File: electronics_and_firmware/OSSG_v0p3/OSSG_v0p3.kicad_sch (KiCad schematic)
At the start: 71 parts, among them IC1 DW01A, J1 USB_B_Micro, J2 External PDM Mic Input, Q1 FS8205A, Q2 Q_NPN_BEC, Q3 Q_NPN_BEC, SW1 SW_SPST, U1 ESP32-PICO-D4, U2 TP4056, U3 XC6222B331MRG, U4 FT232RQ, U5 APX803L-29SA-7, U6 MP23DB01HPTR

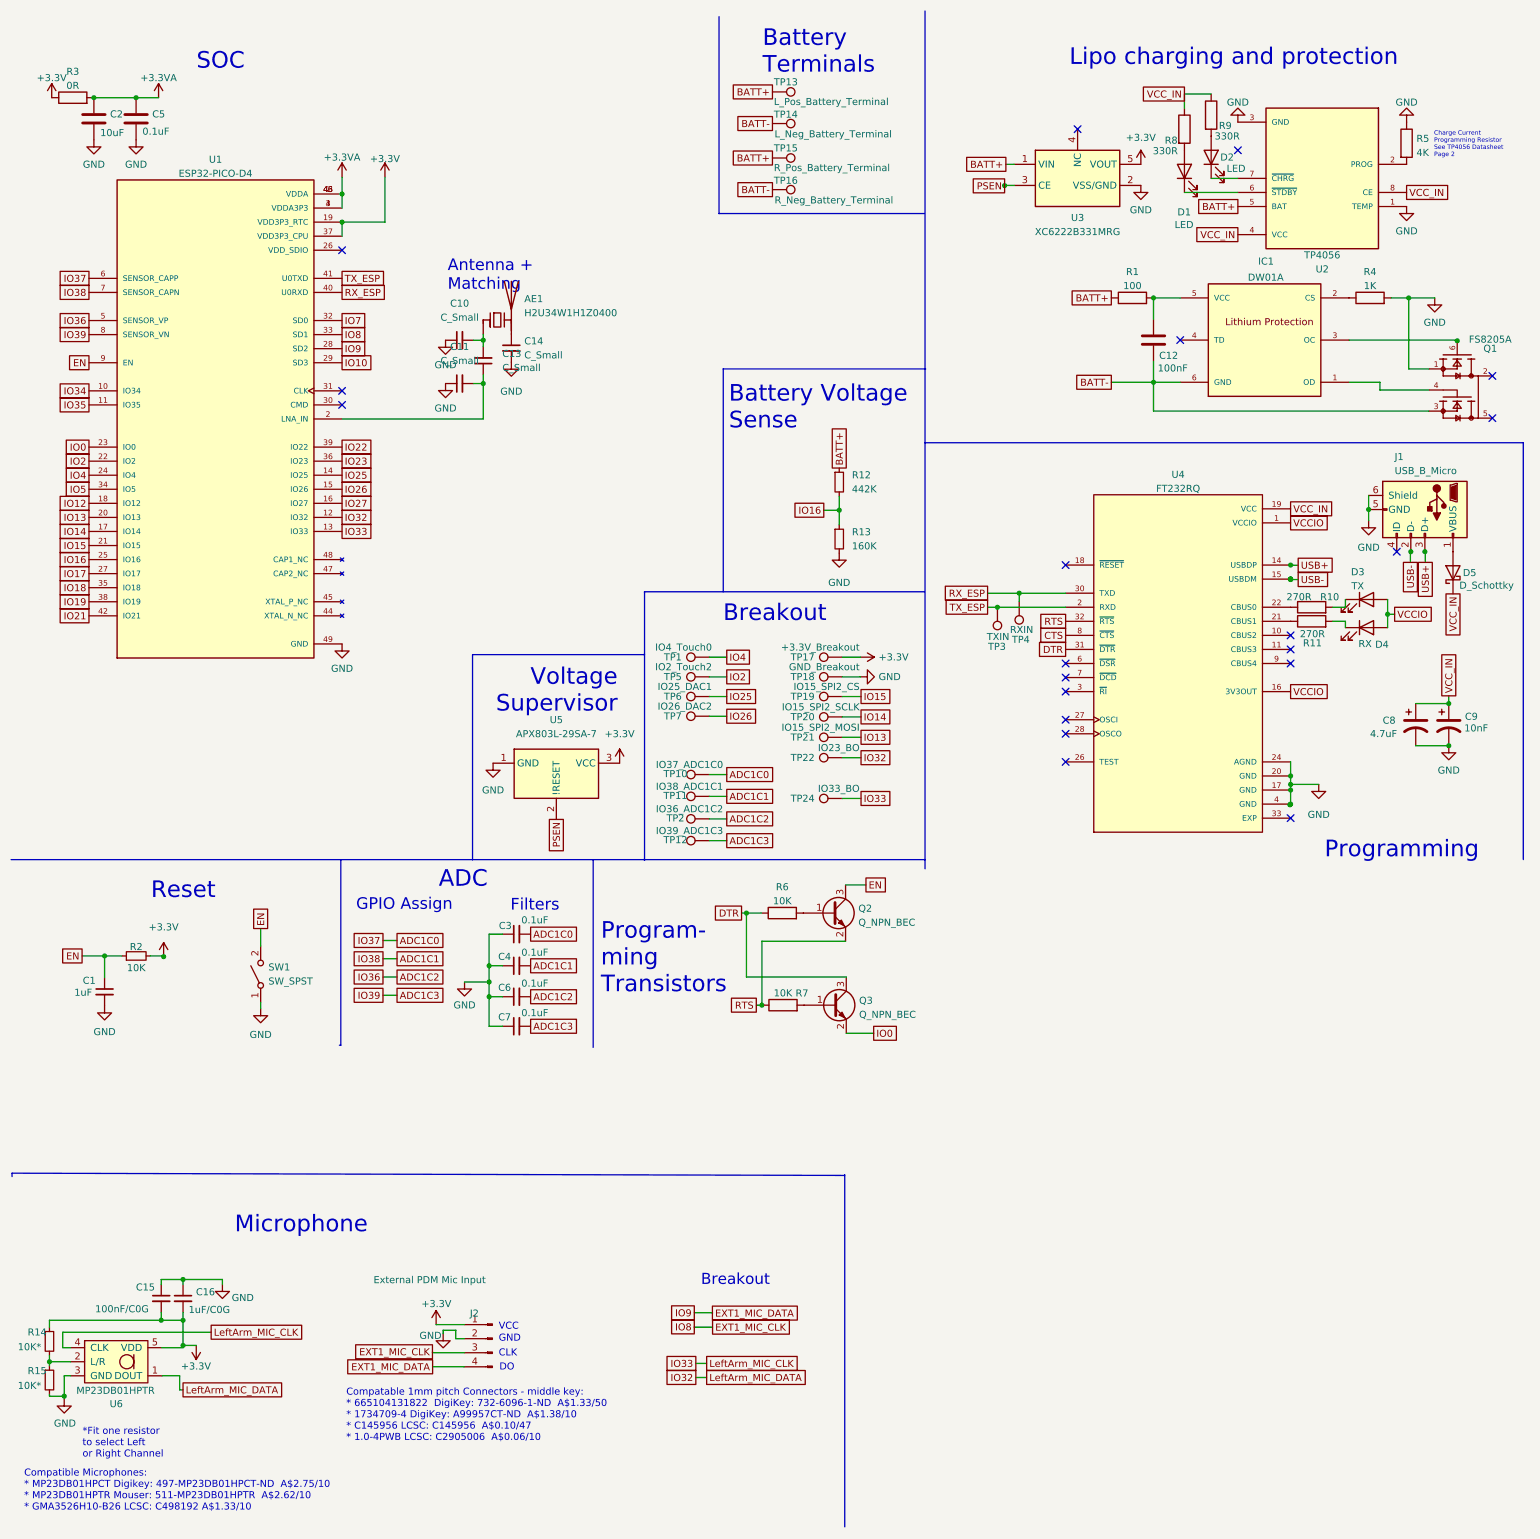
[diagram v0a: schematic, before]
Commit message: Layout and schematic tidying
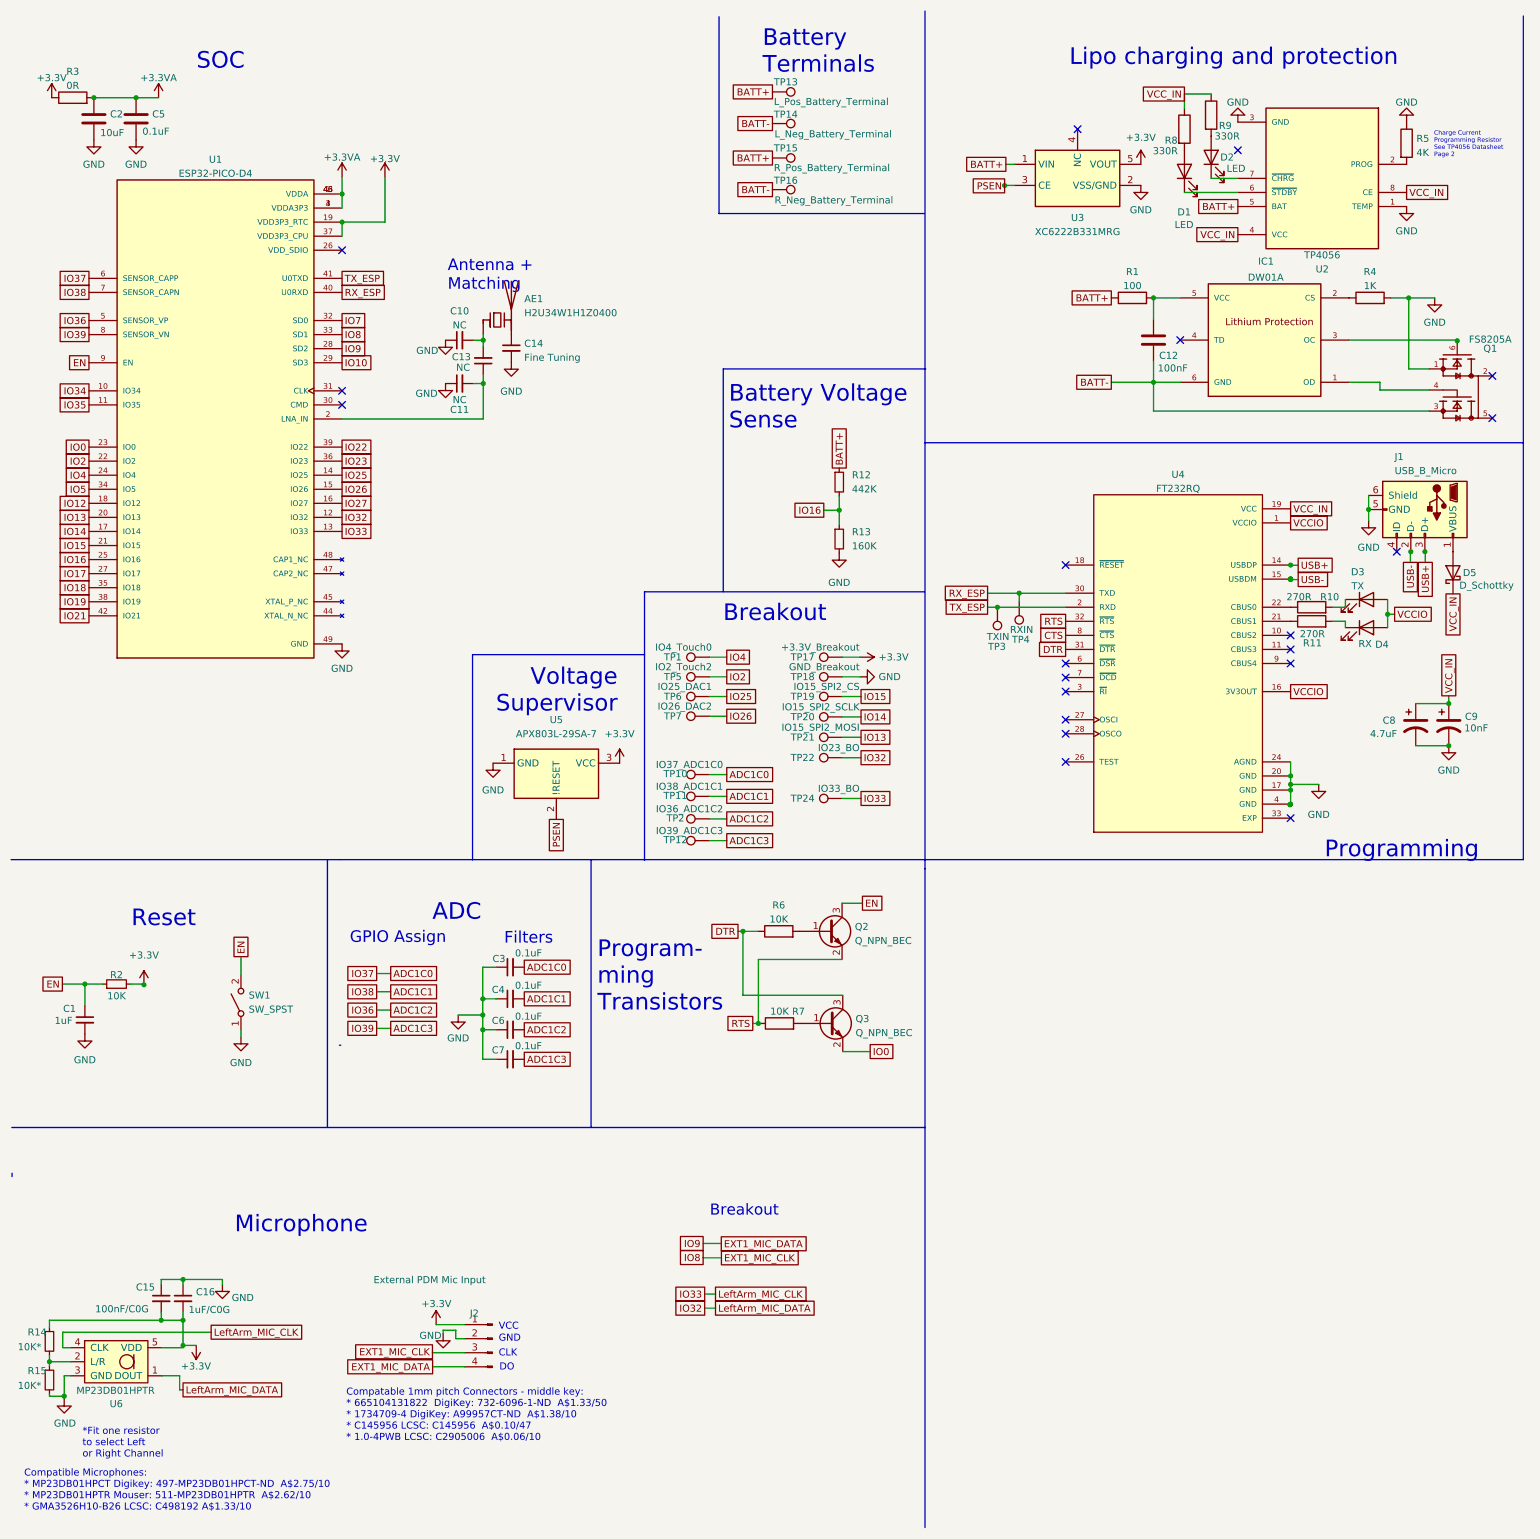
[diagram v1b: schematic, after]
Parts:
- C10, C11, C13: value C_Small -> NC
- C14: value C_Small -> Fine Tuning
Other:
- moved on the sheet: C1, C3, C4, C6, C7, Q2, Q3, R2, R6, R7, SW1
